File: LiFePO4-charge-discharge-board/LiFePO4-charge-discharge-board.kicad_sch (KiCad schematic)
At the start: 10 parts, among them J1 Conn_JST-XH_1x2, J2 mech.-solder-pad_1x2, U1 LiFePO4-Charge

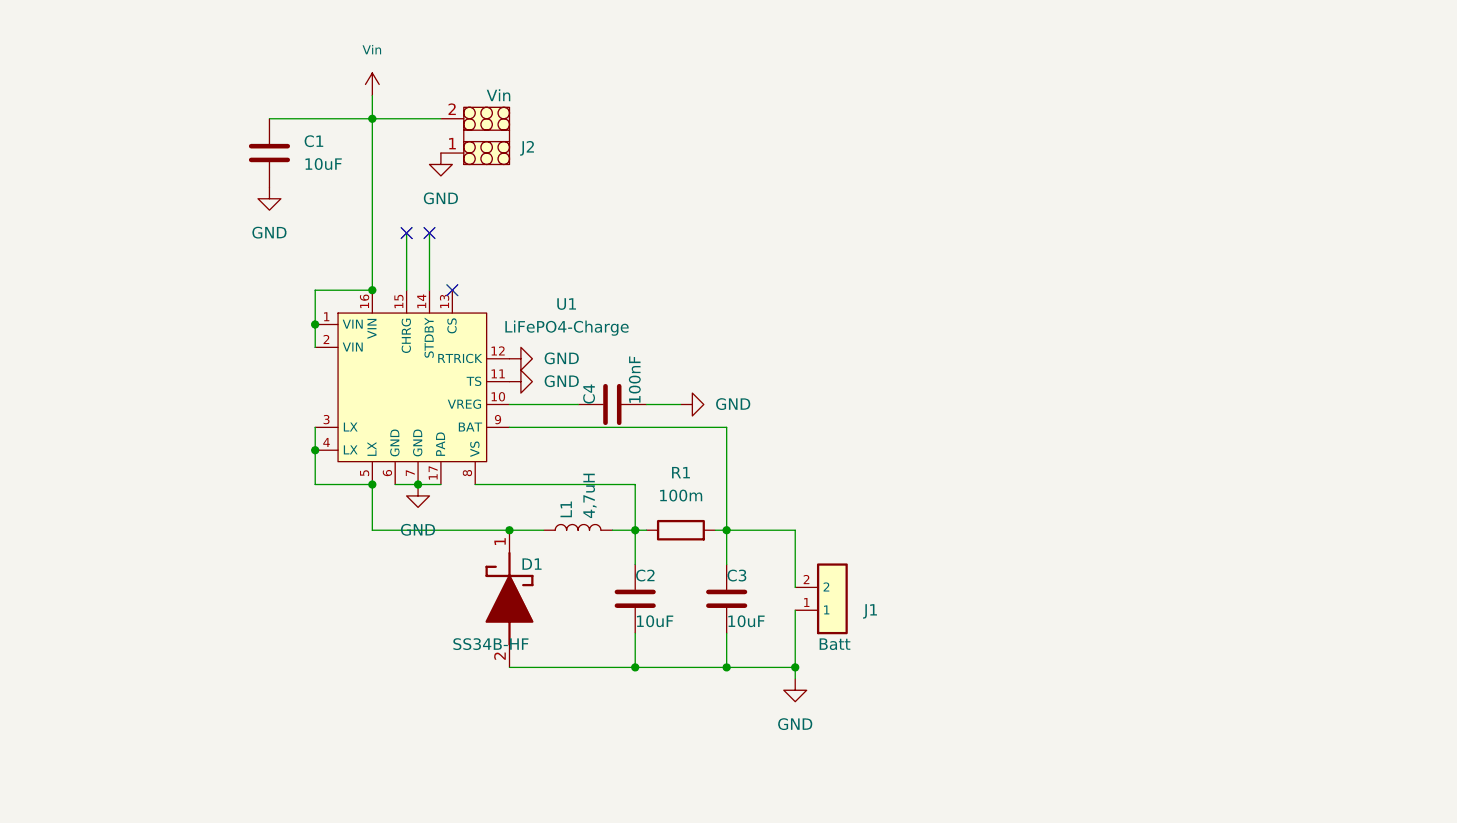
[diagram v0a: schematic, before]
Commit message: rewire circuit
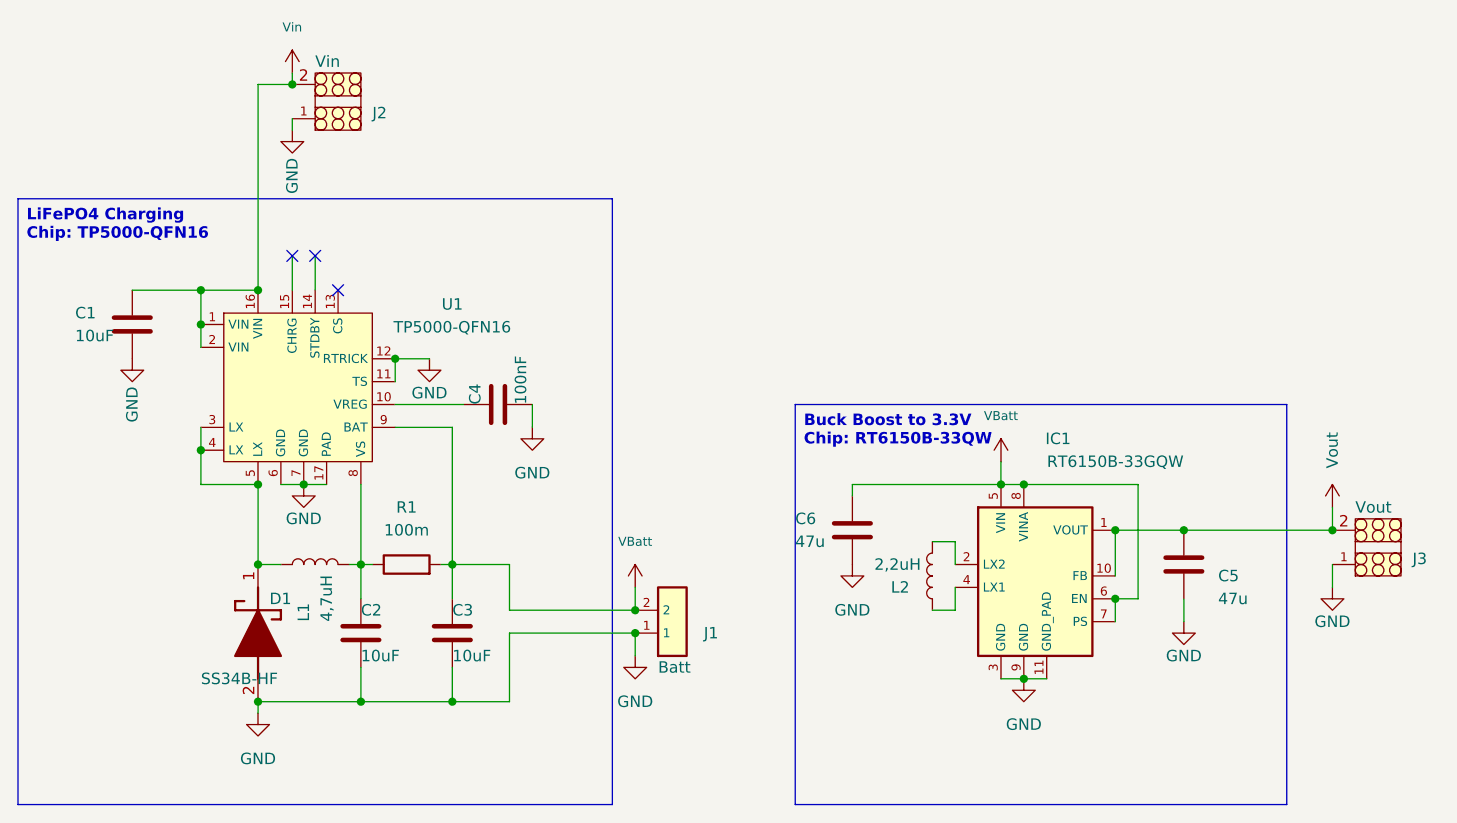
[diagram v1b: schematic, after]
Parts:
- added C5, C6: 47u, Capacitor_SMD:C_0805_2012Metric_Pad1.18x1.45mm_HandSolder, symbol Device:C
- added IC1: RT6150B-33GQW, Marcus-PCB-Library:SON50P250X250X80-11N-D, symbol Marcus-PCB-Library:RT6150B-33GQW
- added J3: mech.-solder-pad_1x2, Marcus-PCB-Library:Conn_Mechc.-solder-pad_1x2, symbol Marcus-PCB-Library:Conn_mech-solder-pad_1x2
- added L2: 2,2uH, Inductor_SMD:L_APV_APH0630, symbol Device:L
- U1: value LiFePO4-Charge -> TP5000-QFN16
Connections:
- net GND: now also C5.2, C6.2, IC1.11 (GND_PAD), IC1.3 (GND), IC1.9 (GND), J3.1
- net VBatt: now reaches C3.1, J1.2, R1.2, U1.9 (BAT)
- net VBatt: now also C6.1, IC1.5 (VIN), IC1.6 (EN), IC1.7 (PS), IC1.8 (VINA)
- new net: IC1.2 (LX2), L2.2
- new net: IC1.4 (LX1), L2.1
- new net Vout: C5.1, IC1.1 (VOUT), IC1.10 (FB), J3.2
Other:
- moved on the sheet: C1, C2, C3, C4, D1, J1, J2, L1, R1, U1

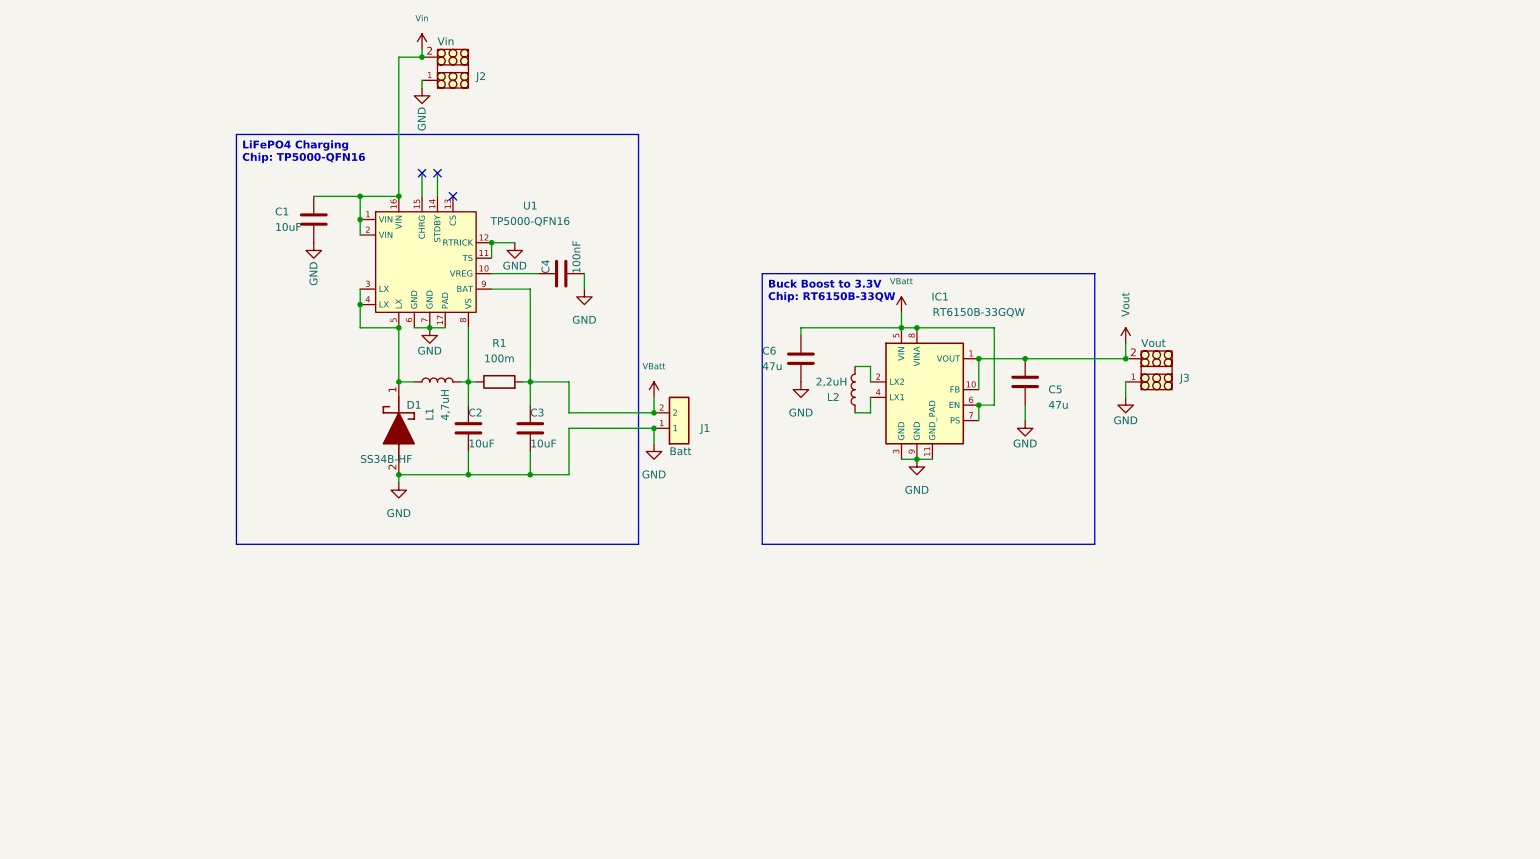
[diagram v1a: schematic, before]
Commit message: Finish version V1.0
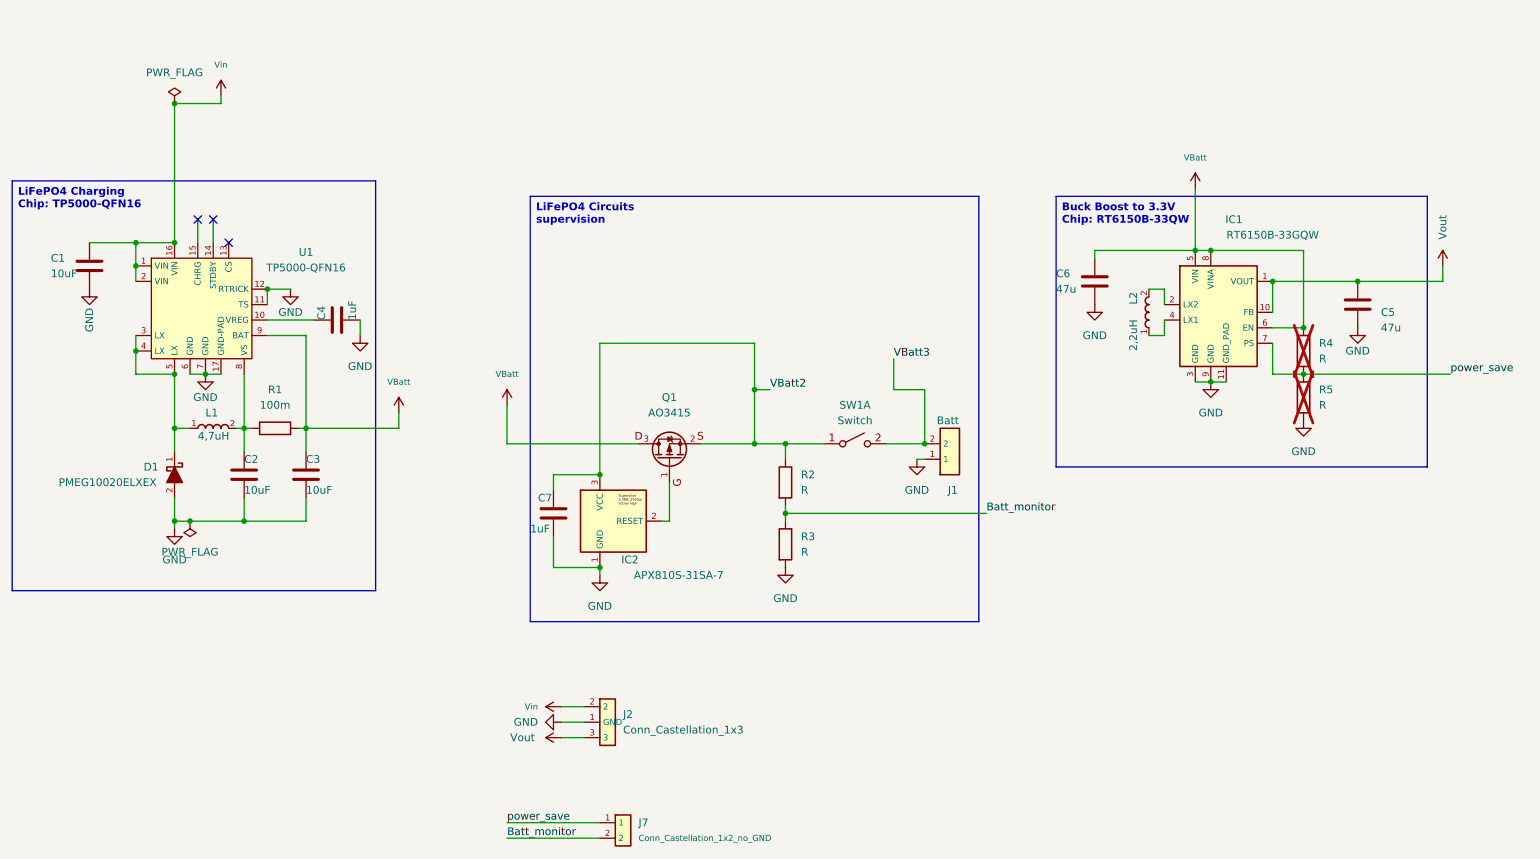
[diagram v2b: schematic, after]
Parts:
- removed D1: SS34B-HF, Marcus-PCB-Library:DIOM5336X320N, symbol Marcus-PCB-Library:SS34B-HF
- removed J2, J3: mech.-solder-pad_1x2, Marcus-PCB-Library:Conn_Mechc.-solder-pad_1x2, symbol Marcus-PCB-Library:Conn_mech-solder-pad_1x2
- removed L2: 2,2uH, Inductor_SMD:L_APV_APH0630, symbol Device:L
- added C7: 1uF, Capacitor_SMD:C_0603_1608Metric, symbol Device:C
- added D1: PMEG10020ELXEX, Marcus_Discretes:PMEG4010EXEX, symbol Marcus_Discretes:PMEG10020ELXEX
- added IC2: APX810S-31SA-7, Marcus_ICs:SOT-23-3_Marcus, symbol Marcus_ICs:APX810S-31SA-7
- added J2: Conn_Castellation_1x3, Marcus_Connectors:Conn_Castellated_1x3_GND_moved, symbol Marcus_Connectors:Conn_Castellation_1x3
- added J7: Conn_Castellation_1x2_no_GND, Marcus_Connectors:Conn_Castellated_1x2_no_GND, symbol Marcus_Connectors:Conn_Castellation_1x2_no_GND
- added L2: 2,2uH, Marcus_Passives:INDC3225X120N, symbol Marcus_Passives:SRP3212A
- added Q1: AO3415, Marcus_ICs:SOT-23-3_Marcus, symbol Marcus_Discretes:AO3415
- added R2, R3, R4, R5: R, Resistor_SMD:R_0603_1608Metric, symbol Device:R
- added SW1: Switch, Marcus_Connectors:Conn_Mechc.-solder-pad_1x2, symbol Switch:SW_DPST_x2
- C1, C2, C3, C5, C6: footprint Capacitor_SMD:C_0805_2012Metric_Pad1.18x1.45mm_HandSolder -> Capacitor_SMD:C_0805_2012Metric
- C4: value 100nF -> 1uF; footprint Capacitor_SMD:C_0805_2012Metric_Pad1.18x1.45mm_HandSolder -> Capacitor_SMD:C_0603_1608Metric
- IC1: footprint Marcus-PCB-Library:SON50P250X250X80-11N-D -> Marcus_ICs:SON50P250X250X80-11N-D; symbol Marcus-PCB-Library:RT6150B-33GQW -> Marcus_ICs:RT6150B-33GQW
- J1: footprint Marcus-PCB-Library:Conn_JST-XH_1x2 -> Marcus_Connectors:Conn_JST-XH_1x2; symbol Marcus-PCB-Library:Conn_JST-XH_1x2 -> Marcus_Connectors:Conn_JST-XH_1x2
- L1: footprint Inductor_SMD:L_APV_APH0630 -> Marcus_Passives:INDC3225X120N; symbol Device:L -> Marcus_Passives:SRP3212A; Height (none) -> 1.2; Manufacturer_Name (none) -> Bourns; Mouser Price/Stock (none) -> https://www.mouser.co.uk/ProductDetail/Bourns/SRP3212A-4R7M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; Series (none) -> SRP3212A
- R1: footprint Resistor_SMD:R_1206_3216Metric_Pad1.30x1.75mm_HandSolder -> Resistor_SMD:R_1206_3216Metric
- U1: footprint Marcus-PCB-Library:TP5000-QFN16 -> Marcus_ICs:TP5000-QFN16; symbol Marcus-PCB-Library:TP5000-QFN16 -> Marcus_ICs:TP5000-QFN16
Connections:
- net GND: now also C7.2, D1.2, IC2.1 (GND), J2.1 (GND), R3.2, R5.2
- net VBatt: now also Q1.3 (D), R4.1; no longer IC1.7 (PS), J1.2
- net Vin: now also J2.2
- net Vout: now also J2.3
- net at L1.1, U1.3 (LX), U1.4 (LX)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: now also D1.1
- net at IC1.2 (LX2): now also L2.2
- net at IC1.4 (LX1): now also L2.1
- new net: IC2.2 (RESET), Q1.1 (G)
- new net Batt_monitor: J7.2, R2.2, R3.1
- new net VBatt2: C7.1, IC2.3 (VCC), Q1.2 (S), R2.1, SW1.1 (A)
- new net VBatt3: J1.2, SW1.2 (B)
- new net power_save: IC1.7 (PS), J7.1, R4.2, R5.1
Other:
- moved on the sheet: C1, C2, C3, C4, C5, C6, IC1, J1, R1, U1
